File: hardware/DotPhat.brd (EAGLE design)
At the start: 30 x 65 mm, 58 parts, among them CN1 1X4-BIG, IC1 CAT24M010TS, IC3 SI1145, J3 USB-MICROB, Q1 BSH103, U1 ATMEGA328P-MU-QFN32, U2 TMP102, U3 ATSHA204-TSU, X2 MC-RTC-RV-4162-C7-I2C, X3 S4B-ZR

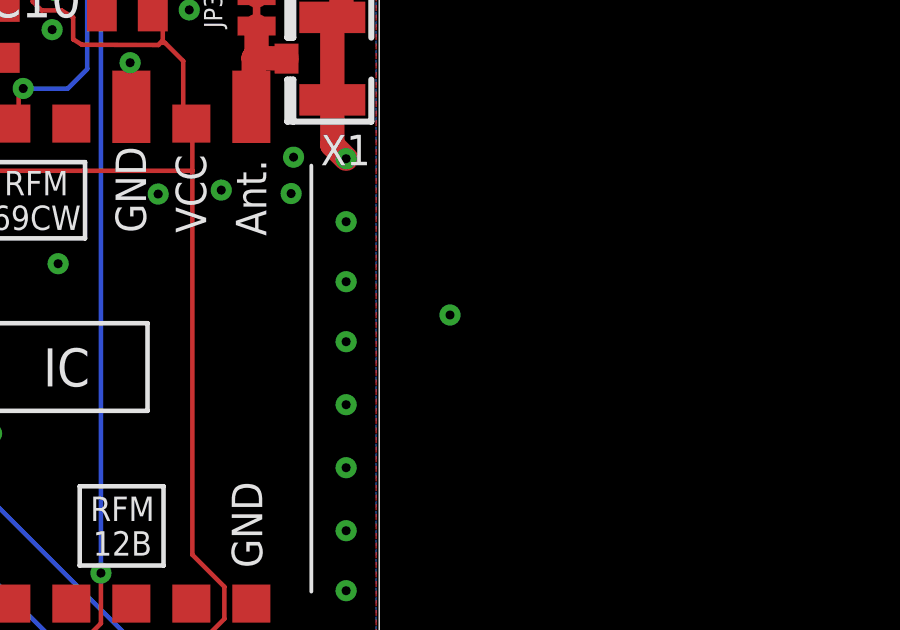
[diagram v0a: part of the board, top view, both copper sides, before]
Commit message: Irrelevant since will be reverted
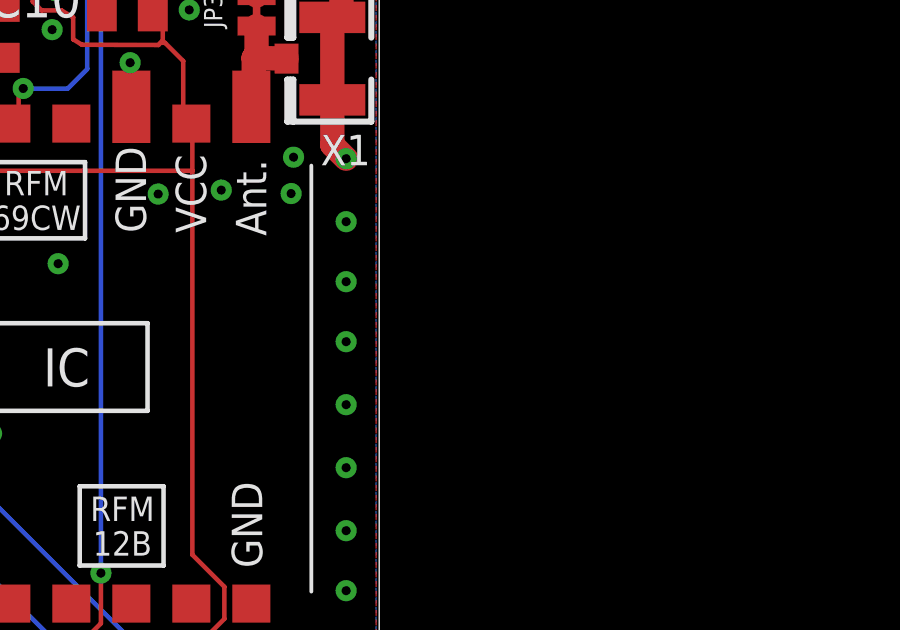
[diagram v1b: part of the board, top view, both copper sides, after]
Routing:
- net GND: vias 145 -> 144
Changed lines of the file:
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@@
 <via x="5.489240625" y="15.109725" extent="1-16" drill="0.3"/>
 <via x="5.743240625" y="24.828725" extent="1-16" drill="0.3"/>
-<via x="32.362240625" y="14.089725" extent="1-16" drill="0.3"/>
 <via x="1.967240625" y="7.861725" extent="1-16" drill="0.3"/>
 <via x="3.920240625" y="9.865725" extent="1-16" drill="0.3"/>
@@
 <contactref element="C11" pad="-"/>
 <contactref element="JP5" pad="2"/>
-<wire x1="28.9" y1="13.2" x2="32.362240625" y2="14.089725" width="0" layer="19" extent="1-1"/>
 </signal>
 <signal name="SDA">

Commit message: Revert "Irrelevant since will be reverted"
This reverts commit e891d672a37a9ace9540b21aee4dc257b77b94d6.
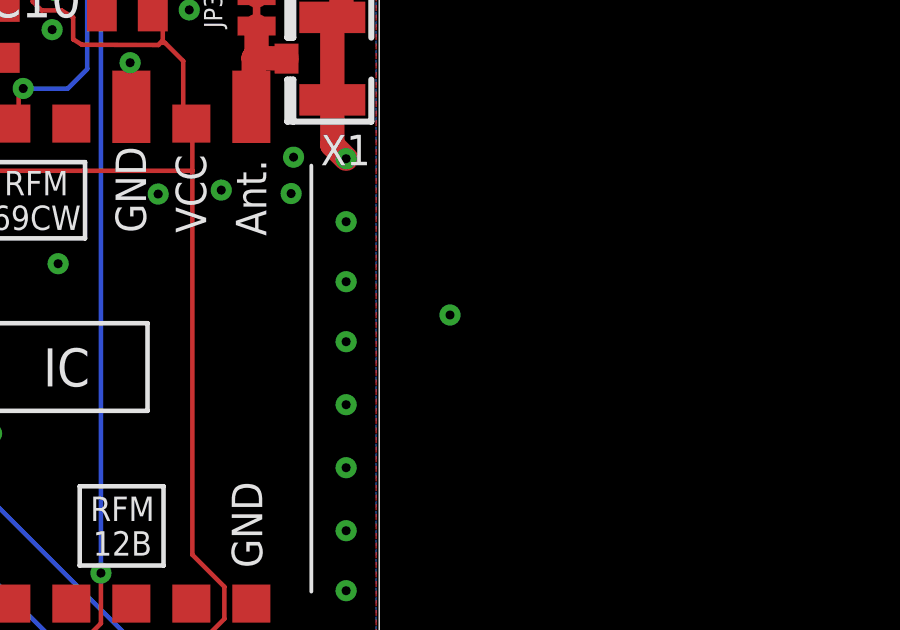
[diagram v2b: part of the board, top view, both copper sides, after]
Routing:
- net GND: vias 144 -> 145
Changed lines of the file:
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@@
 <via x="5.489240625" y="15.109725" extent="1-16" drill="0.3"/>
 <via x="5.743240625" y="24.828725" extent="1-16" drill="0.3"/>
+<via x="32.362240625" y="14.089725" extent="1-16" drill="0.3"/>
 <via x="1.967240625" y="7.861725" extent="1-16" drill="0.3"/>
 <via x="3.920240625" y="9.865725" extent="1-16" drill="0.3"/>
@@
 <contactref element="C11" pad="-"/>
 <contactref element="JP5" pad="2"/>
+<wire x1="28.9" y1="13.2" x2="32.362240625" y2="14.089725" width="0" layer="19" extent="1-1"/>
 </signal>
 <signal name="SDA">
